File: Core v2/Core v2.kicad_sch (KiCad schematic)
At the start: 49 parts, among them CN1 PJ-3200, J1 Serial Debug, J2 USB_C_Receptacle_USB2.0, Q1 BSS138, SW1 SW_SPST, SW2 SW_SPST, SW3 SW_SPST, U1 DL-TX1-433M, U2 H34B-433M, U3 ESP32-S3-WROOM-1, U4 MCP1700x-300xxTT, U5 AMS1117-3.3

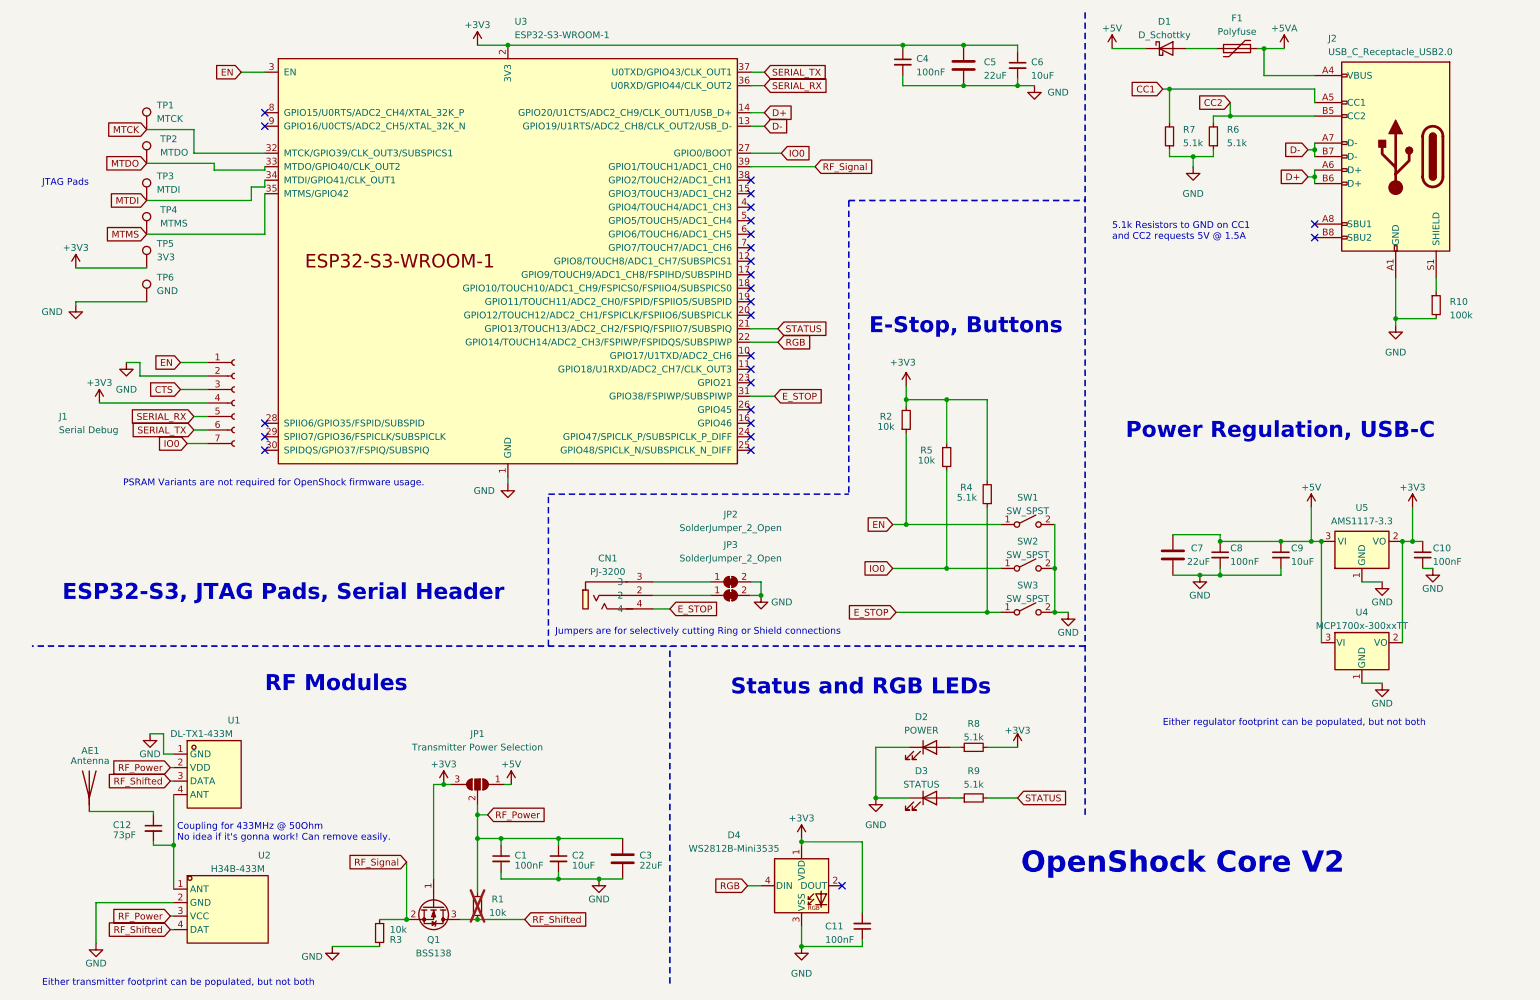
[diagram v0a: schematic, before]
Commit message: Core V2.1 KiCad + JLC Files
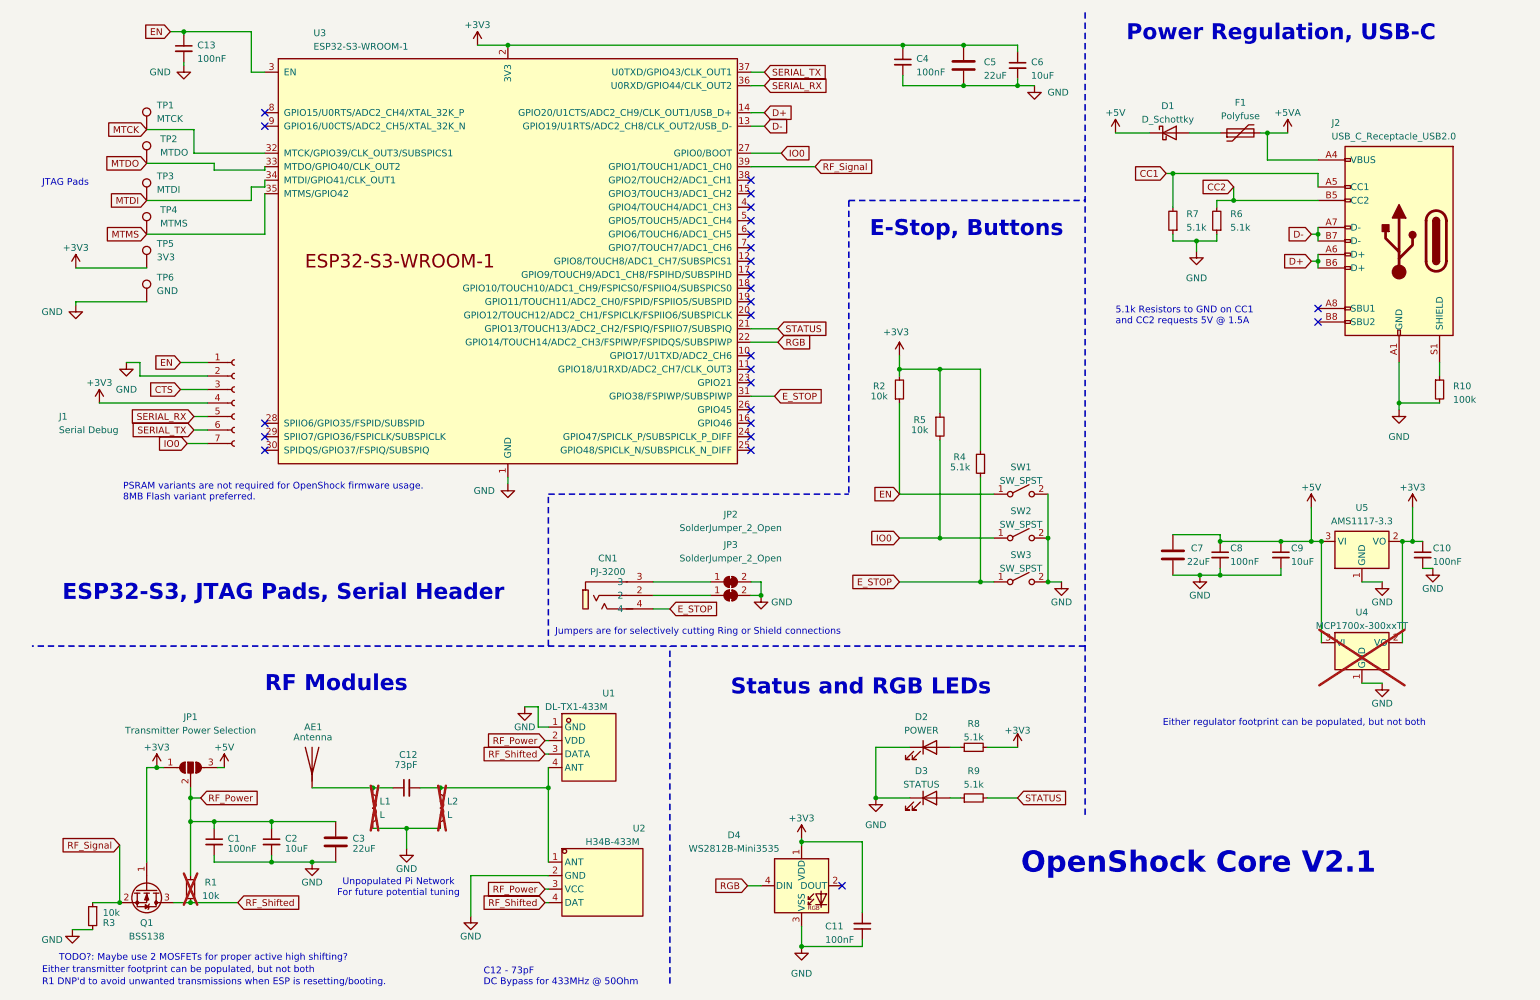
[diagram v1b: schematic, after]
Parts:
- added C13: 100nF, Capacitor_SMD:C_0603_1608Metric_Pad1.08x0.95mm_HandSolder, symbol Device:C_Small
- added L1, L2: L, Inductor_SMD:L_0603_1608Metric_Pad1.05x0.95mm_HandSolder, symbol Device:L
- AE1: footprint Connector_PinHeader_2.54mm:PinHeader_1x01_P2.54mm_Vertical -> Connector_Pin:Pin_D1.0mm_L10.0mm
- J1, JP1, JP2, JP3, R1, TP1, TP2, TP3, TP4, TP5, TP6: now left out of the parts list
- U4: now not fitted; now left out of the parts list
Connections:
- net +3V3: now also JP1.1 (A); no longer JP1.3 (B)
- net +5V: now also JP1.3 (B); no longer JP1.1 (A)
- net EN: now also C13.1
- net GND: now also C13.2, L1.2, L2.2
- net at C12.2, U1.4 (ANT), U2.1 (ANT): now also L2.1
- net at AE1.1 (A), C12.1: now also L1.1
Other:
- note added: "C12 - 73pF DC Bypass for 433MHz @ 50Ohm"
- note added: "OpenShock Core V2.1"
- note added: "PSRAM variants are not required for OpenShock firmware usage. 8MB Flash variant preferred."
- note added: "R1 DNP'd to avoid unwanted transmissions when ESP is resetting/booting."
- note added: "TODO?: Maybe use 2 MOSFETs for proper active high shifting?"
- note added: "Unpopulated Pi Network For future potential tuning"
- note removed: "Coupling for 433MHz @ 50Ohm No idea if it's gonna work! Can remove easily."
- note removed: "OpenShock Core V2"
- note removed: "PSRAM Variants are not required for OpenShock firmware usage."
- moved on the sheet: AE1, C1, C12, C2, C3, D1, F1, J2, JP1, Q1, R1, R10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

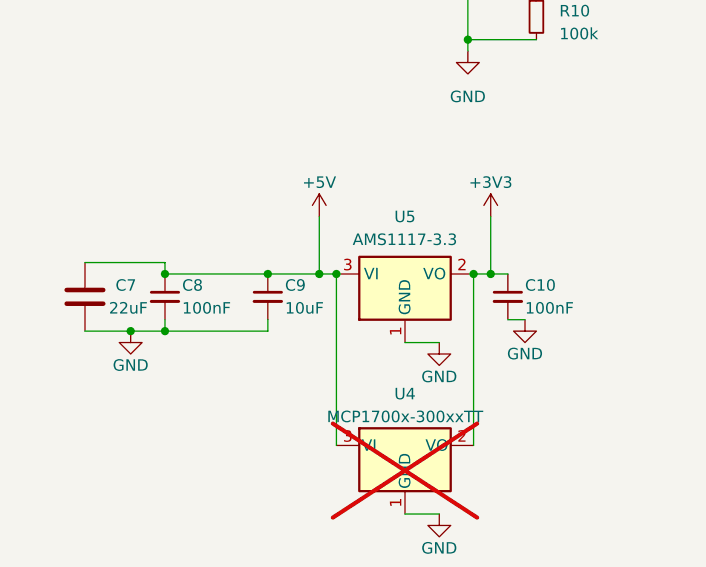
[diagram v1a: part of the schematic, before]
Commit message: Core V2.2 KiCad + JLC Files
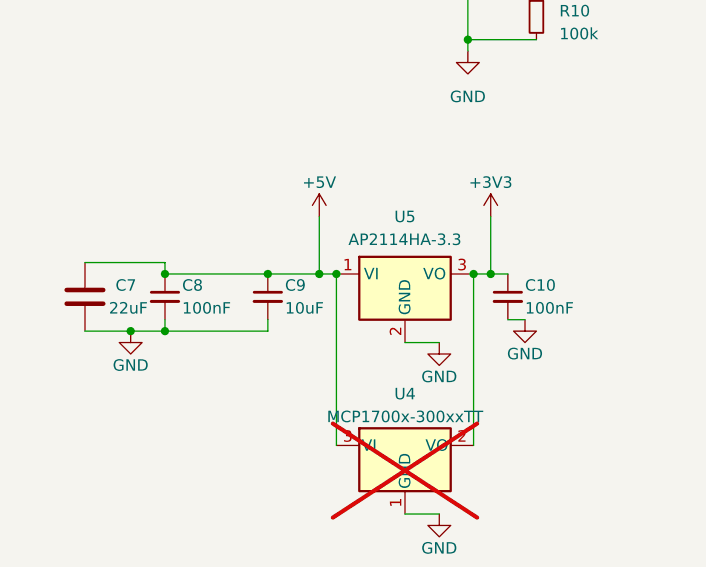
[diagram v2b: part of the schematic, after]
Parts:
- U5: value AMS1117-3.3 -> AP2114HA-3.3
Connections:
- net +3V3: now also U5.3 (VO); no longer U5.2 (VO)
- net +5V: now also U5.1 (VI); no longer U5.3 (VI)
- net GND: now also U5.2 (GND); no longer U5.1 (GND)
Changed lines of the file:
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@@
 			)
 		)
-		(property "Value" "AMS1117-3.3"
+		(property "Value" "AP2114HA-3.3"
 			(at 262.255 109.855 0)
 			(effects
@@
 			)
 		)
-		(property "Datasheet" "http://www.advanced-monolithic.com/pdf/ds1117.pdf"
+		(property "Datasheet" "https://wmsc.lcsc.com/wmsc/upload/file/pdf/v2/lcsc/2304140030_Diodes-Incorporated-AP2114HA-3-3TRG1_C460314.pdf"
 			(at 264.795 120.015 0)
 			(effects
